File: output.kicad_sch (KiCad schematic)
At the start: 29 parts

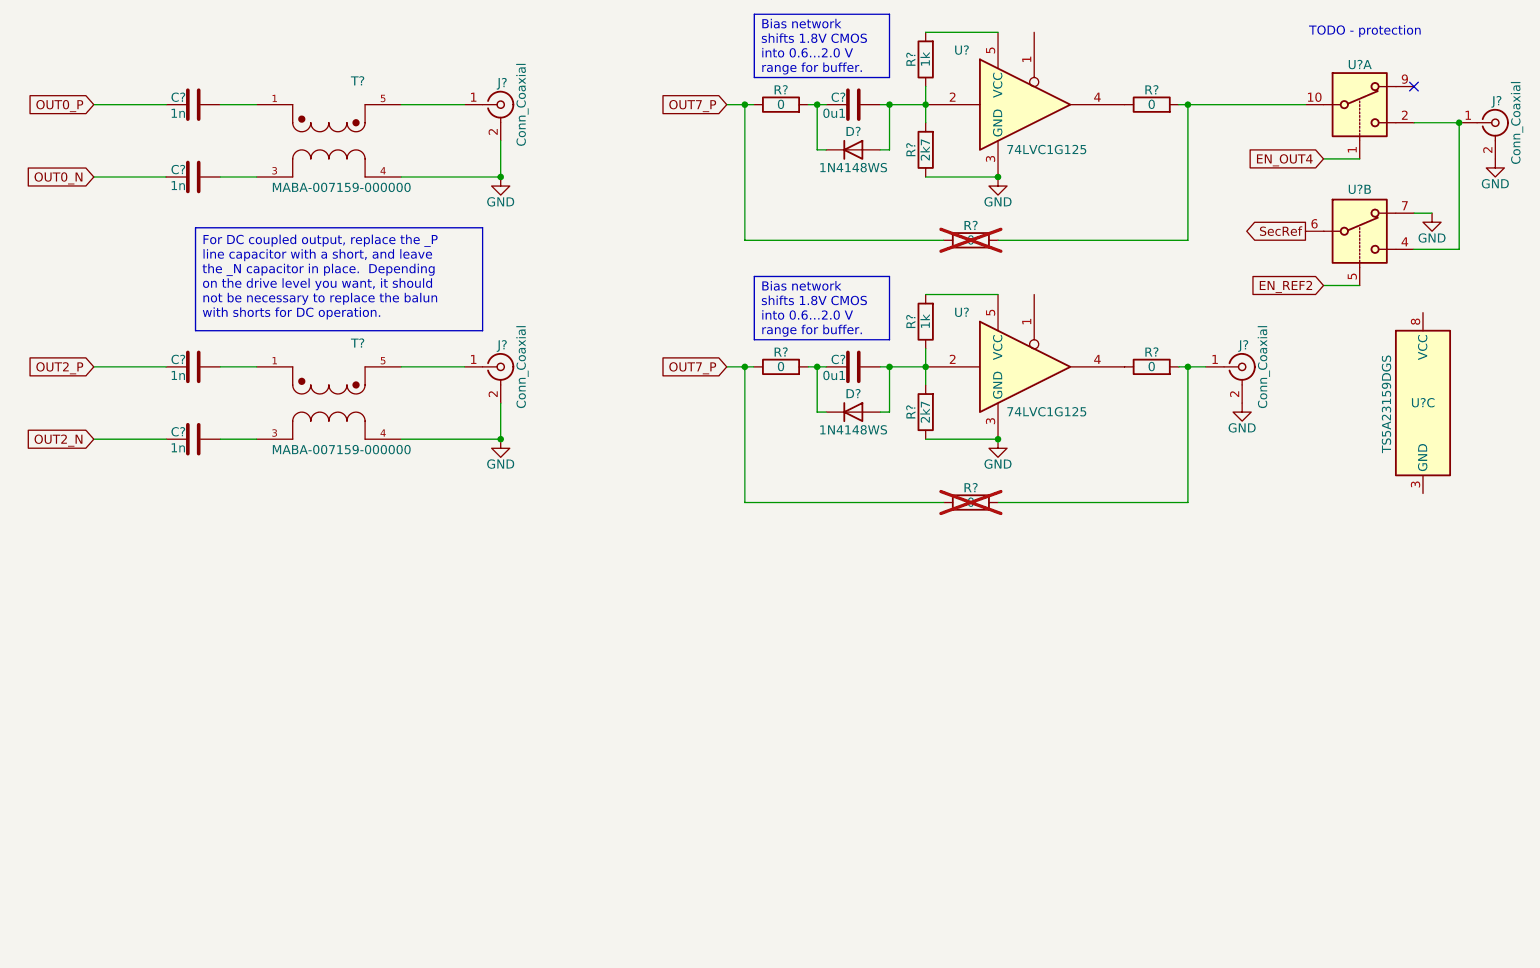
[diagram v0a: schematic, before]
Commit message: Schematic is basically feature complete
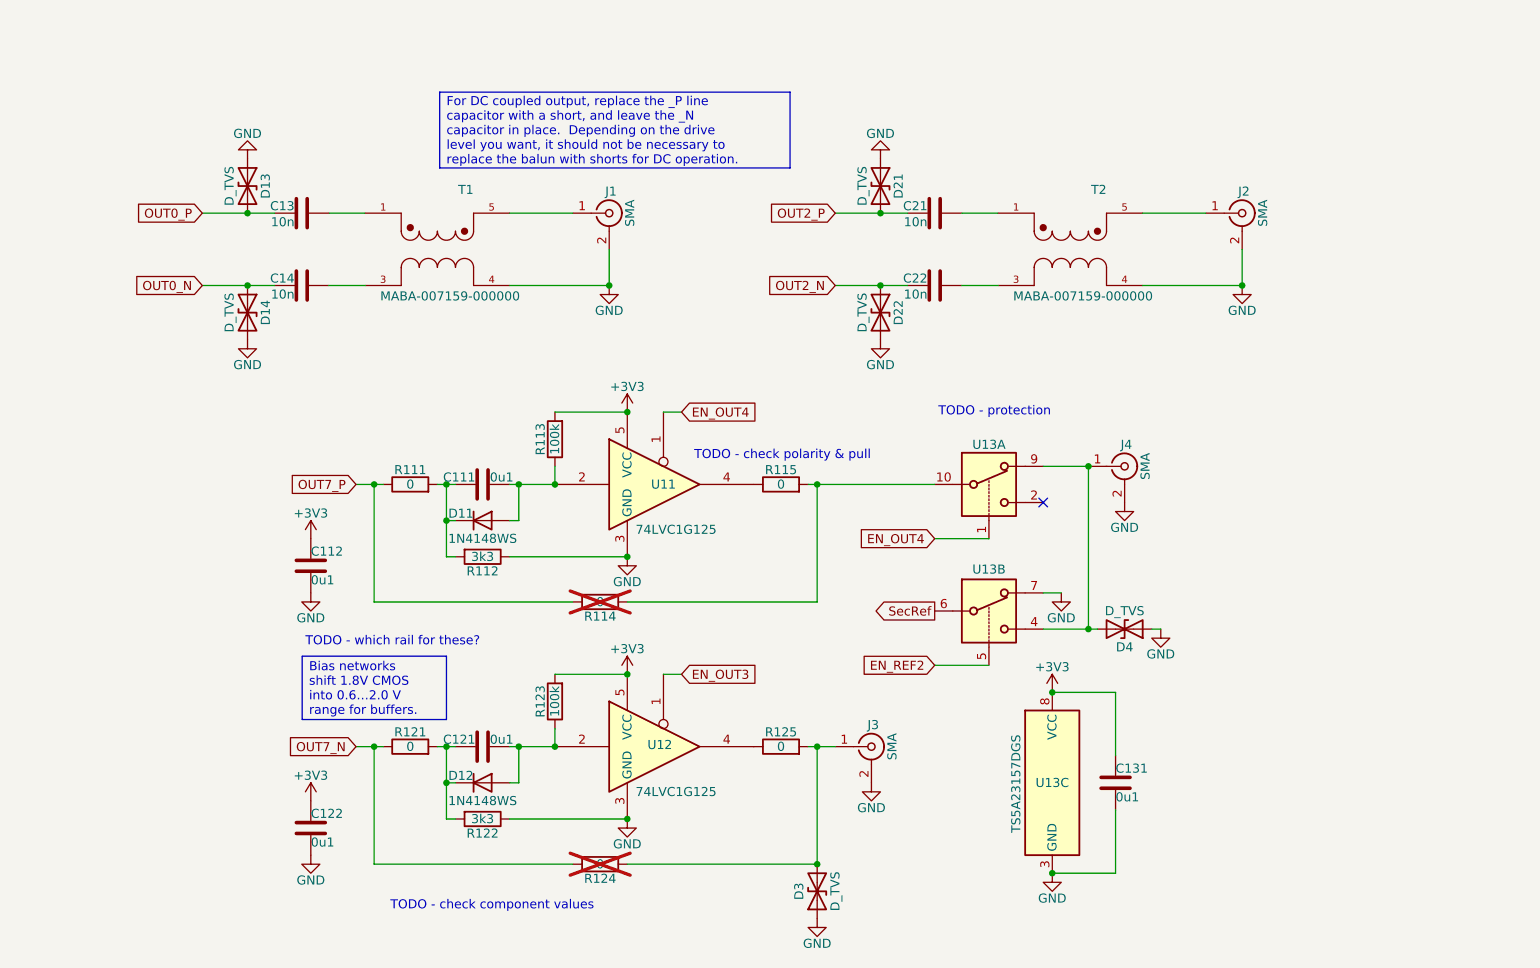
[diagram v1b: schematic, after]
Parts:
- added C112, C122, C131: 0u1, Capacitor_SMD:C_0402_1005Metric, symbol Device:C
- added D13, D14, D21, D22, D3, D4: D_TVS, Diode_SMD:D_0402_1005Metric_Pad0.77x0.64mm_HandSolder, symbol Device:D_TVS
- C13, C14, C21, C22: renamed from C?; value 1n -> 10n
- J1, J2, J3, J4: renamed from J?; value Conn_Coaxial -> SMA; now left out of the parts list
- R112, R122: renamed from R?; value 2k7 -> 3k3
- R113, R123: renamed from R?; value 1k -> 100k
- T1, T2: renamed from T?; MANUFACTURER M/A-Com Technology Solutions -> (none); PARTREV v5 -> (none); STANDARD Manufacturer Recommendations -> (none)
- U11, U12: renamed from U?; footprint (none) -> Package_TO_SOT_SMD:SOT-353_SC-70-5; now left out of the parts list
- U13: renamed from U?; value TS5A23159DGS -> TS5A23157DGS; now left out of the parts list
- gave numbers to parts that had none: 10
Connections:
- net EN_OUT4: now also U11.1
- net GND: now also U13.3 (GND), C112.2, C122.2, C131.2, D13.1 (A1), D14.2 (A2), D21.1 (A1), D22.2 (A2), D3.1 (A1), D4.1 (A1)
- net OUT0_N: now also D14.1 (A1)
- net OUT0_P: now also D13.2 (A2)
- net OUT2_N: now also D22.1 (A1)
- net OUT2_P: now also D21.2 (A2)
- net OUT7_P: no longer R121.1, R124.1
- net at J4.1 (In), U13.4: now also U13.9, D4.2 (A2); no longer U13.2
- net at C121.1, D12.1 (K), R121.2: now also R122.2
- net at C121.2, D12.2 (A), R123.1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: no longer R122.2
- net EN_OUT3: now reaches U12.1
- net +3V3: now reaches R123.2, U12.5 (VCC)
- net +3V3: now also R113.2, U11.5 (VCC), U13.8 (VCC), C112.1, C122.1, C131.1
- net at J3.1 (In), R124.2, R125.2: now also D3.2 (A2)
- net at C111.1, D11.1 (K), R111.2: now also R112.2
- net at C111.2, D11.2 (A), R113.1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: no longer R112.2
- new net OUT7_N: R121.1, R124.1
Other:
- note added: "TODO - check component values"
- note added: "TODO - check polarity & pull"
- note added: "TODO - which rail for these?"
- moved on the sheet: C111, C121, C13, C14, C21, C22, D11, D12, J1, J2, J3, J4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
